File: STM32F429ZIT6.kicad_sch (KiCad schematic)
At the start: 115 parts, among them J1 Conn_02x24_Odd_Even, J2 Conn_01x05_Pin, J3 Conn_02x16_Odd_Even, SW1 K3-1235S, U2 LD3985M33R, U3 MCP6004, U4 NAU88C22YG_C914209, U5 RCLAMP0521P.TCT_C3029033, U6 RCLAMP0521P.TCT_C3029033, U7 W9825G6KH-6, X1 7V25000014

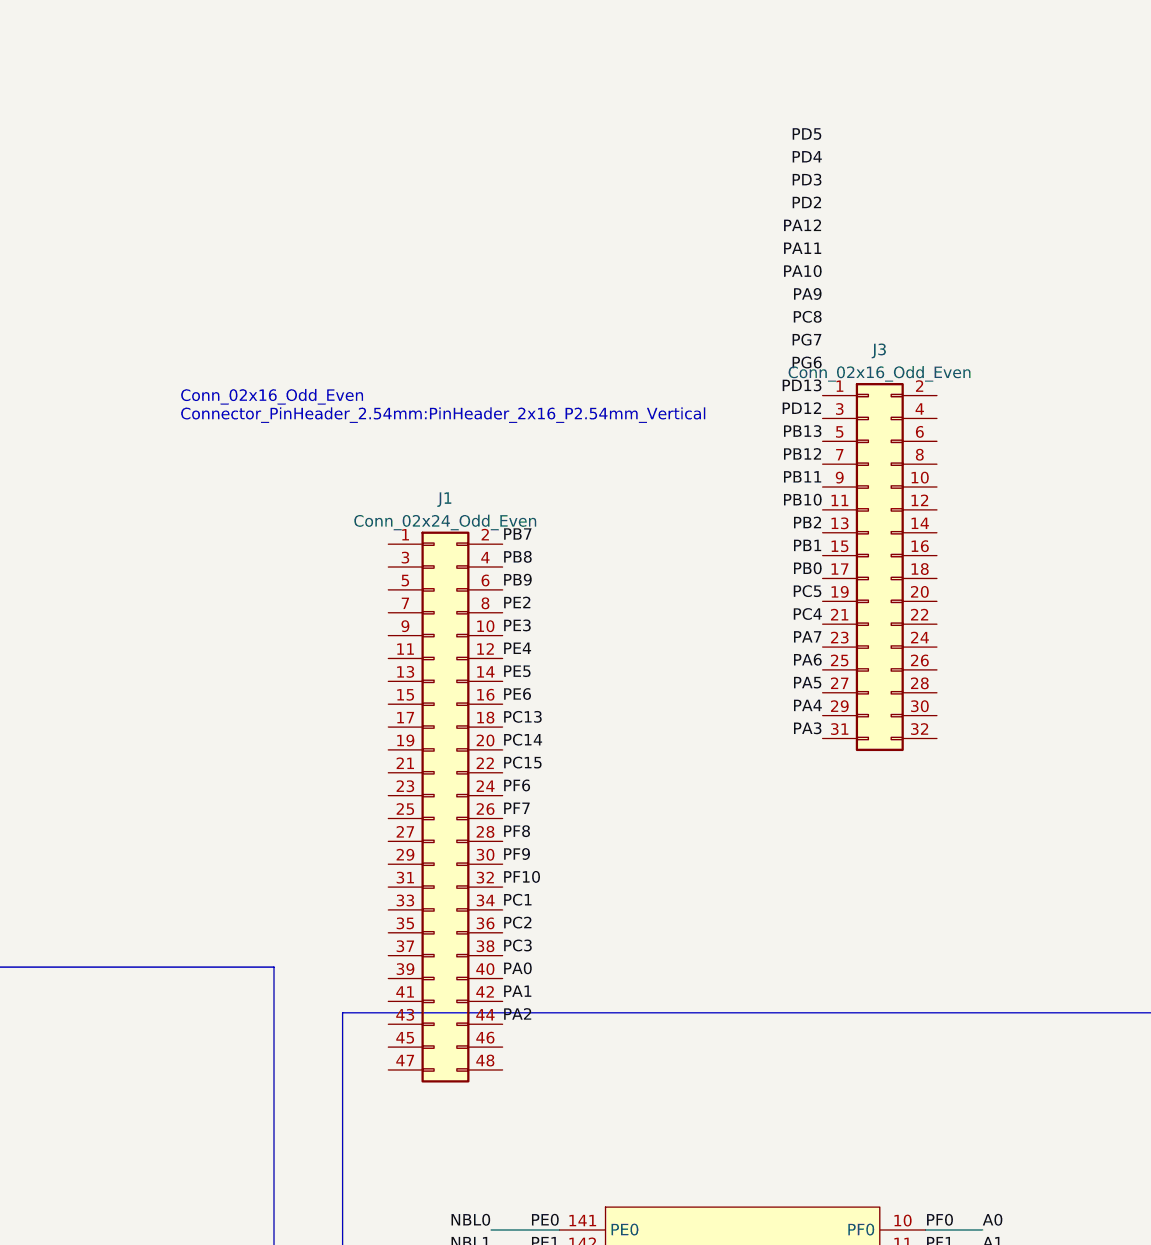
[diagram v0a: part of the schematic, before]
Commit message: quick save
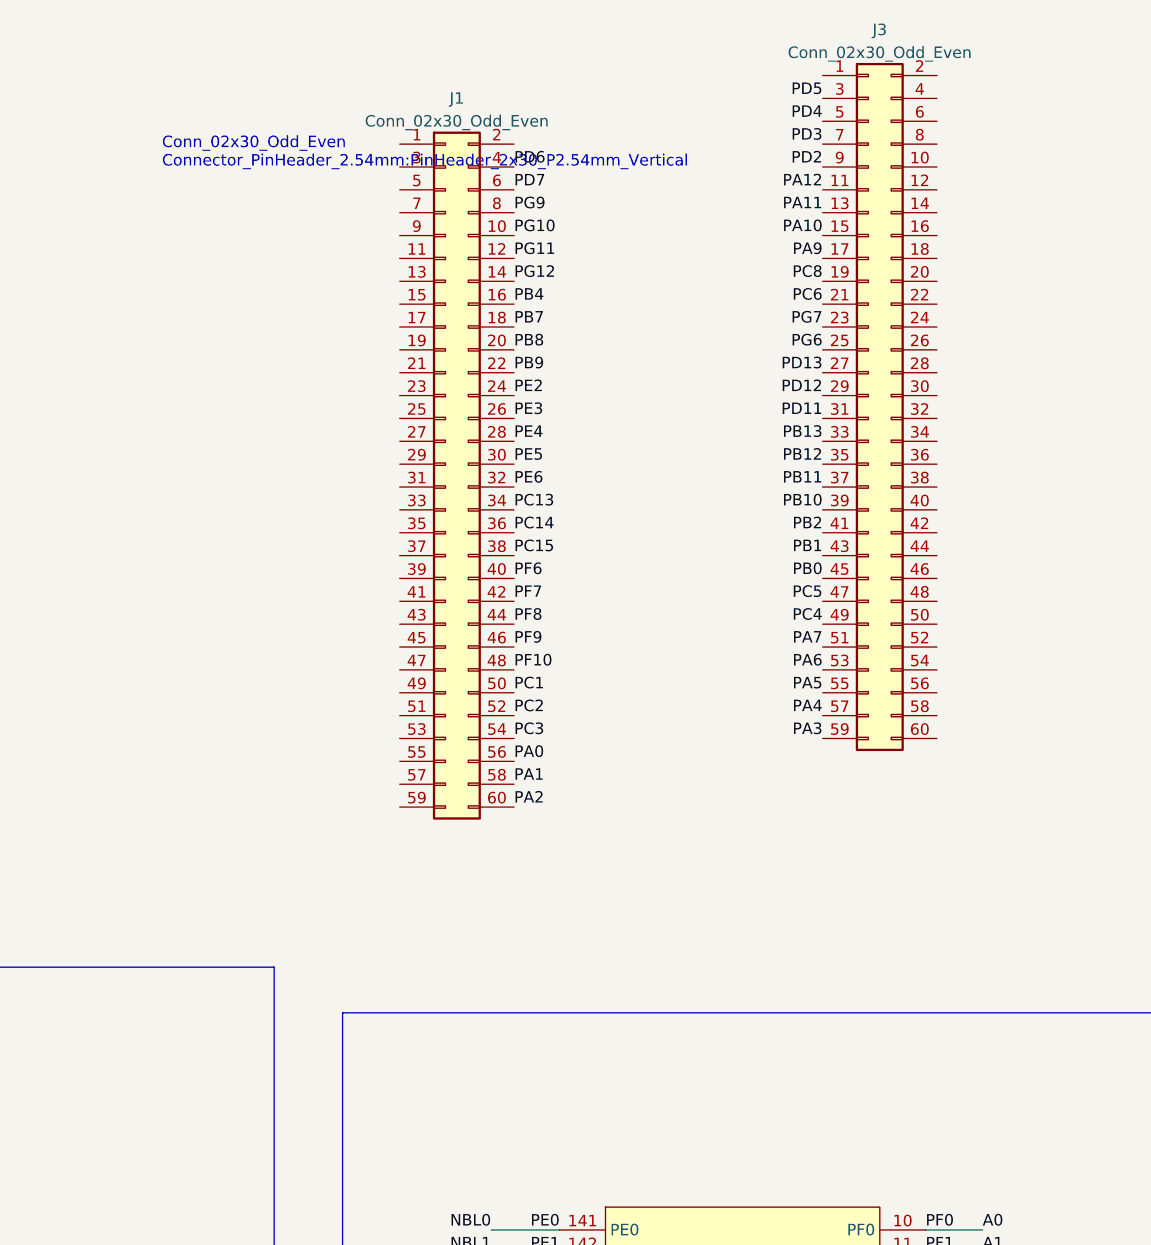
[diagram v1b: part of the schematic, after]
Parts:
- removed J1: Conn_02x24_Odd_Even, Connector_PinHeader_2.54mm:PinHeader_2x24_P2.54mm_Vertical, symbol Connector_Generic:Conn_02x24_Odd_Even
- removed J3: Conn_02x16_Odd_Even, Connector_PinHeader_2.54mm:PinHeader_2x16_P2.54mm_Vertical, symbol Connector_Generic:Conn_02x16_Odd_Even
- added J1, J3: Conn_02x30_Odd_Even, Connector_PinHeader_2.54mm:PinHeader_2x30_P2.54mm_Vertical, symbol Connector_Generic:Conn_02x30_Odd_Even
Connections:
- net PA0: now also J1.56 (Pin_56)
- net PA1: now also J1.58 (Pin_58)
- net PA10: now also J3.15 (Pin_15)
- net PA11: now also J3.13 (Pin_13)
- net PA12: now also J3.11 (Pin_11)
- net PA2: now also J1.60 (Pin_60)
- net PA3: now also J3.59 (Pin_59)
- net PA4: now also J3.57 (Pin_57)
- net PA5: now also J3.55 (Pin_55)
- net PA6: now also J3.53 (Pin_53)
- net PA7: now also J3.51 (Pin_51)
- net PA9: now also J3.17 (Pin_17)
- net PB0: now also J3.45 (Pin_45)
- net PB1: now also J3.43 (Pin_43)
- net PB10: now also J3.39 (Pin_39)
- net PB11: now also J3.37 (Pin_37)
- net PB12: now also J3.35 (Pin_35)
- net PB13: now also J3.33 (Pin_33)
- net PB2: now also J3.41 (Pin_41)
- net PB4: now also J1.16 (Pin_16)
- net PB7: now also J1.18 (Pin_18)
- net PB8: now also J1.20 (Pin_20)
- net PB9: now also J1.22 (Pin_22)
- net PC1: now also J1.50 (Pin_50)
- net PC13: now also J1.34 (Pin_34)
- net PC14: now also J1.36 (Pin_36)
- net PC15: now also J1.38 (Pin_38)
- net PC2: now also J1.52 (Pin_52)
- net PC3: now also J1.54 (Pin_54)
- net PC4: now also J3.49 (Pin_49)
- net PC5: now also J3.47 (Pin_47)
- net PC6: now also J3.21 (Pin_21)
- net PC8: now also J3.19 (Pin_19)
- net PD11: now also J3.31 (Pin_31)
- net PD12: now also J3.29 (Pin_29)
- net PD13: now also J3.27 (Pin_27)
- net PD2: now also J3.9 (Pin_9)
- net PD3: now also J3.7 (Pin_7)
- net PD4: now also J3.5 (Pin_5)
- net PD5: now also J3.3 (Pin_3)
- net PD6: now also J1.4 (Pin_4)
- net PD7: now also J1.6 (Pin_6)
- net PE2: now also J1.24 (Pin_24)
- net PE3: now also J1.26 (Pin_26)
- net PE4: now also J1.28 (Pin_28)
- net PE5: now also J1.30 (Pin_30)
- net PE6: now also J1.32 (Pin_32)
- net PF10: now also J1.48 (Pin_48)
- net PF6: now also J1.40 (Pin_40)
- net PF7: now also J1.42 (Pin_42)
- net PF8: now also J1.44 (Pin_44)
- net PF9: now also J1.46 (Pin_46)
- net PG10: now also J1.10 (Pin_10)
- net PG11: now also J1.12 (Pin_12)
- net PG12: now also J1.14 (Pin_14)
- net PG6: now also J3.25 (Pin_25)
- net PG7: now also J3.23 (Pin_23)
- net PG9: now also J1.8 (Pin_8)
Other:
- note added: "Conn_02x30_Odd_Even Connector_PinHeader_2.54mm:PinHeader_2x30_P2.54mm_Vertical"
- note removed: "Conn_02x16_Odd_Even Connector_PinHeader_2.54mm:PinHeader_2x16_P2.54mm_Vertical"
